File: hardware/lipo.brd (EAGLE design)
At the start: 33.5 x 34.6 mm, 50 parts, among them J1 MICRO_USB_B_HIROSE_ZX62-B-5PA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, Q1 IRLML6402, Q2 IRLML6344, SW1 TVAF06-A020B-R, U1 LT6106CS5#PBF, U2 NJM12888F, X1 FA-238

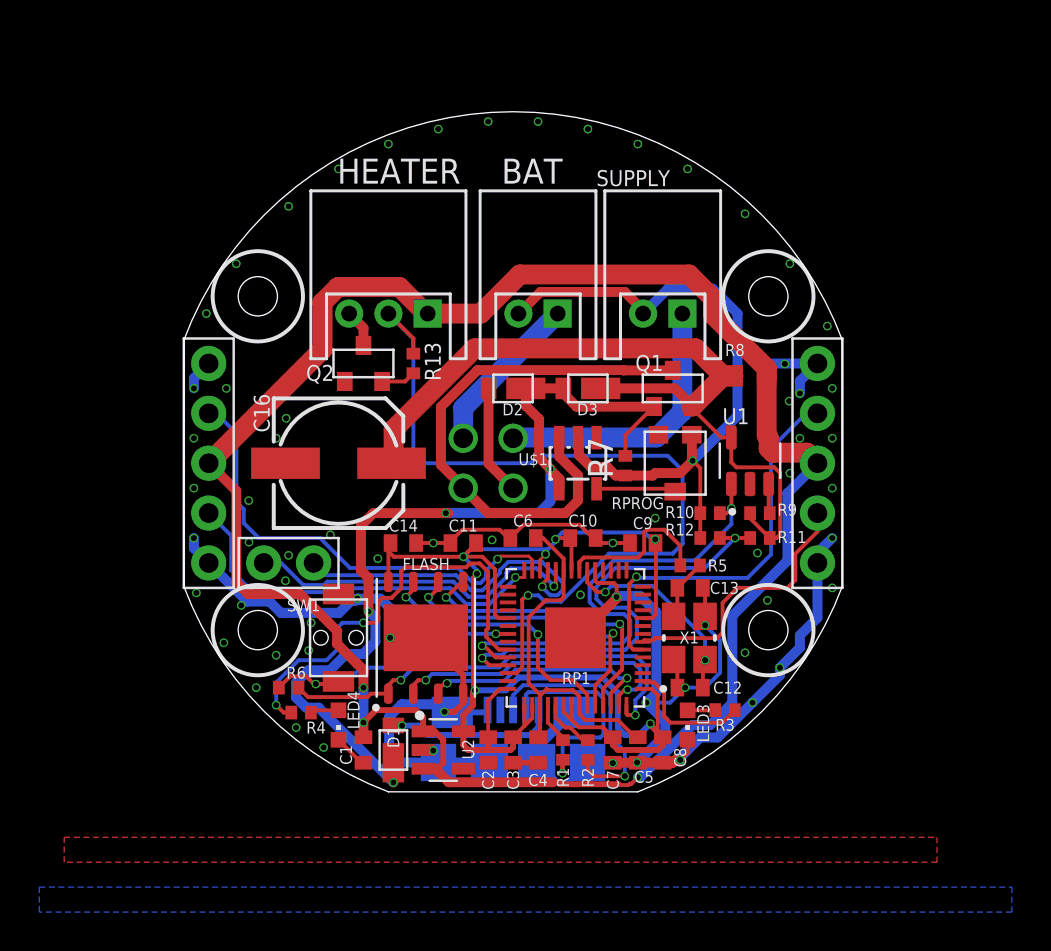
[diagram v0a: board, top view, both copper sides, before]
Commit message: 微修正
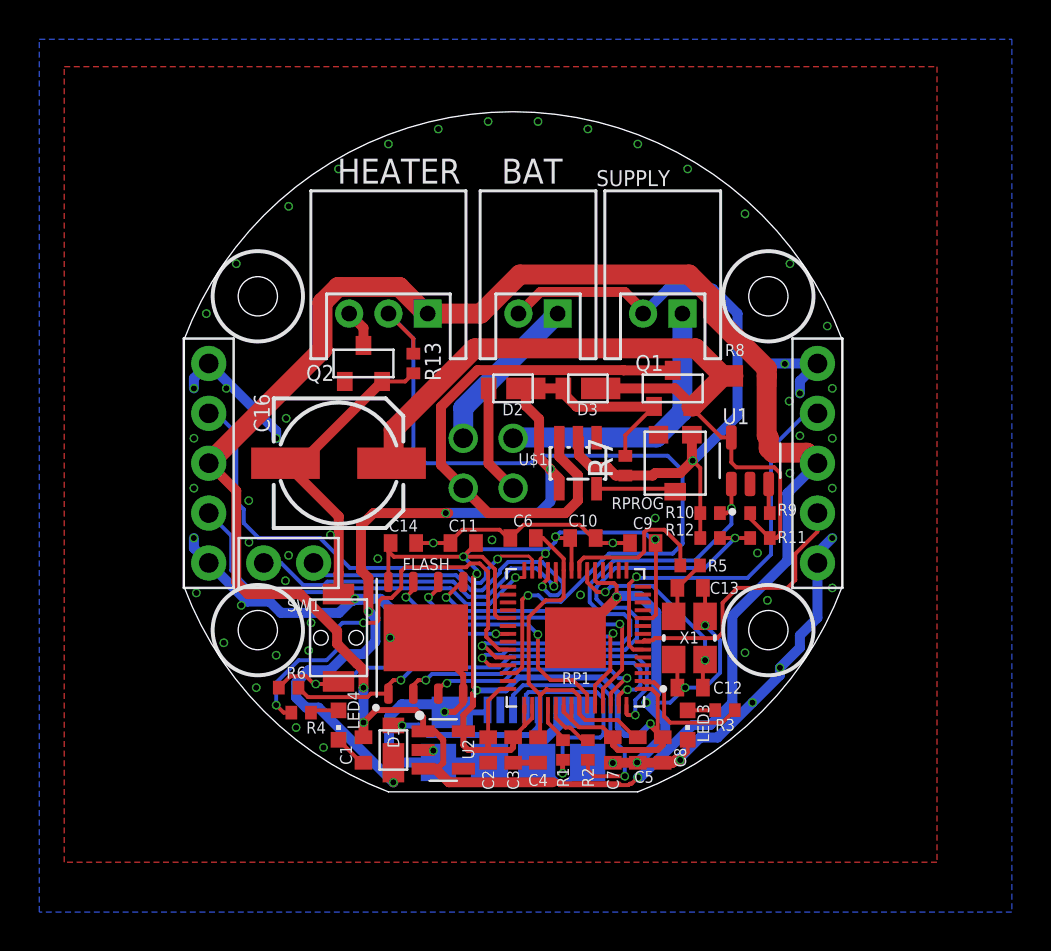
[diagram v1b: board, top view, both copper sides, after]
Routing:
- net GND: track 155.3 -> 175.0 mm
